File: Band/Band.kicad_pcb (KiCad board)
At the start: 2 copper layers, 24 x 22.5 mm, 32 parts, among them U1 ESP32-C3-WROOM-02, U2 TC2014-1.8VxCTTR, U3 BMP280, U4 BMI270, U5 MAX30102, U6 BQ25504, U7 S-1318A33

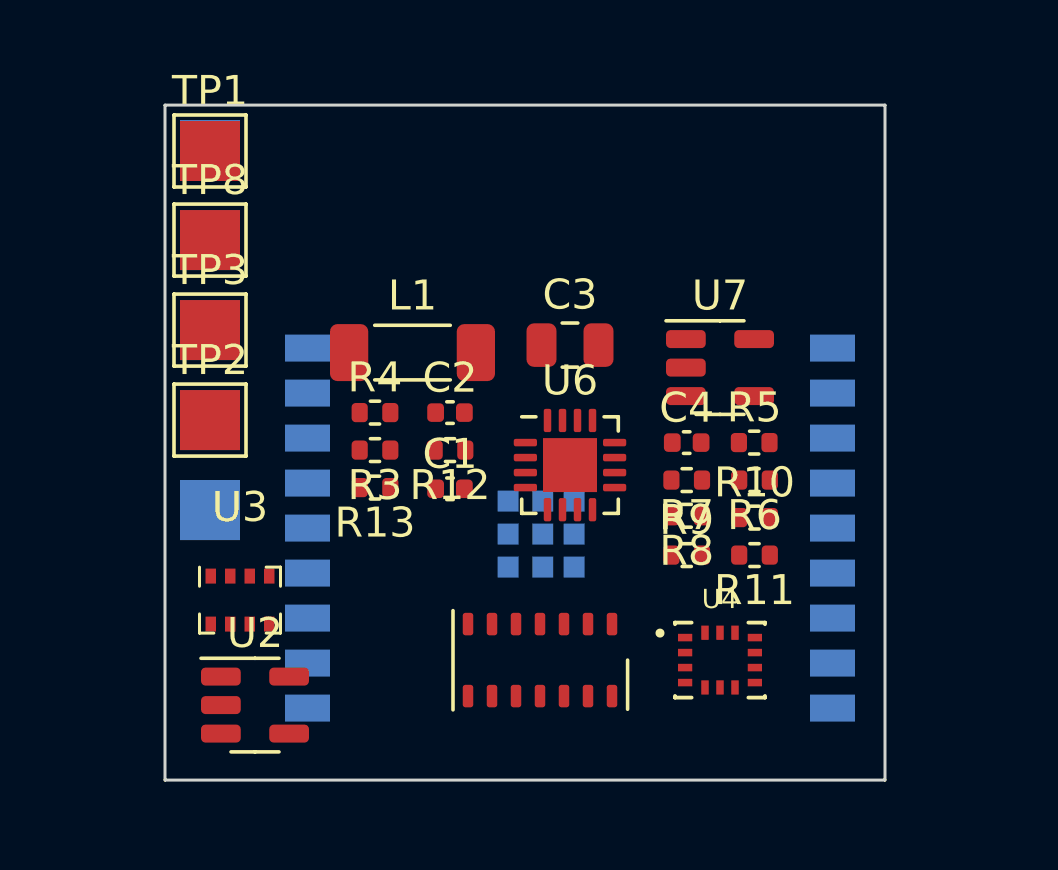
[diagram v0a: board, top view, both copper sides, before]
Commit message: finish layout and route
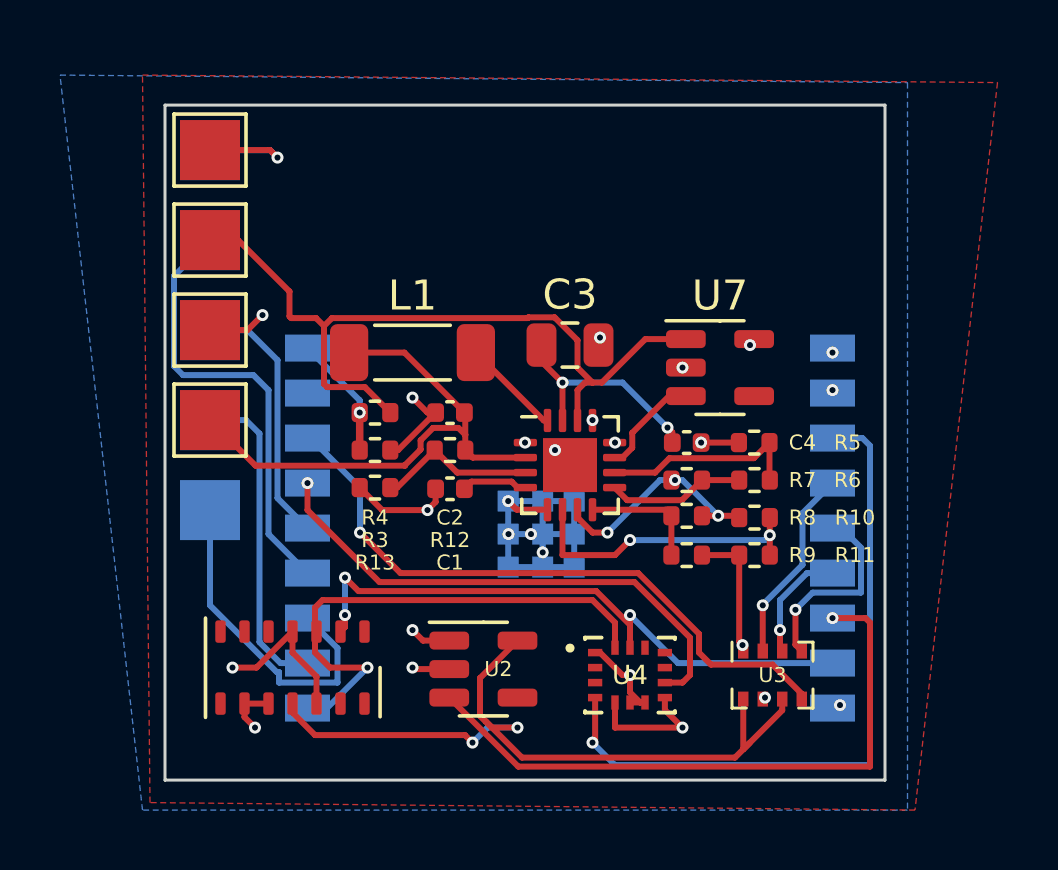
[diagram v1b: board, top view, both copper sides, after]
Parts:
- moved U3 17.9 mm to (184.2, 62.0)
- moved U5 8.25 mm to (168.2, 61.8)
- moved U2 7.71 mm to (174.6, 61.8)
- moved U4 3.04 mm to (179.5, 62.0)
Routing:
- net GND: track 0.00 -> 42.7 mm, vias 0 -> 21
- net Net-(U2-Pad5): track 0.00 -> 26.5 mm, vias 0 -> 2
- net /Power_Management/BATT: track 0.00 -> 25.8 mm
- net Net-(U1-Pad3): track 0.00 -> 23.1 mm, vias 0 -> 1
- net SPI_MISO: track 0.00 -> 21.4 mm, vias 0 -> 1
- net Net-(U1-Pad7): track 0.00 -> 21.1 mm, vias 0 -> 1
- net SCL: track 0.00 -> 20.9 mm, vias 0 -> 3
- net /Power_Management/PV: track 0.00 -> 18.0 mm
- net Net-(U1-Pad15): track 0.00 -> 17.6 mm, vias 0 -> 1
- net SDA: track 0.00 -> 17.3 mm, vias 0 -> 1
- net Net-(U1-Pad13): track 0.00 -> 14.8 mm
- net Net-(TP7-Pad1): track 0.00 -> 11.3 mm
- net Net-(TP5-Pad1): track 0.00 -> 10.7 mm
- net Net-(R10-Pad2): track 0.00 -> 9.95 mm, vias 0 -> 2
- net Net-(U1-Pad14): track 0.00 -> 8.68 mm
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- added copper zone on B.Cu, net +3.3V
- added copper zone on In1.Cu, net +3.3V
- added copper zone on F.Cu, net GND
- added copper zone on In2.Cu, net GND
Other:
- copper layers 2 -> 4
